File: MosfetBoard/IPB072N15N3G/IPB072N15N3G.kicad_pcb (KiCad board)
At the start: 2 copper layers, 147 x 100 mm, 94 parts, among them J1 DRIVER1, J13 BATT+Conn2, J14 BATT-Conn2, J2 DRIVER1, J3 DRIVER1, J4 PhaseConn, J5 PhaseConn, J6 PhaseConn, J8 BATT+Conn1, J9 BATT-Conn1, Q1 IPB072N15N3G, Q10 IPB072N15N3G, Q11 IPB072N15N3G, Q12 IPB072N15N3G, Q2 IPB072N15N3G, Q3 IPB072N15N3G, Q4 IPB072N15N3G, Q5 IPB072N15N3G, Q6 IPB072N15N3G, Q7 IPB072N15N3G, Q8 IPB072N15N3G, Q9 IPB072N15N3G, U1 RS2166XC5, U2 ACS773ECB-200B-PFF-T, U3 ACS773ECB-200B-PFF-T, U5 RS2166XC5, U6 ACS773ECB-200B-PFF-T, U7 RS2166XC5

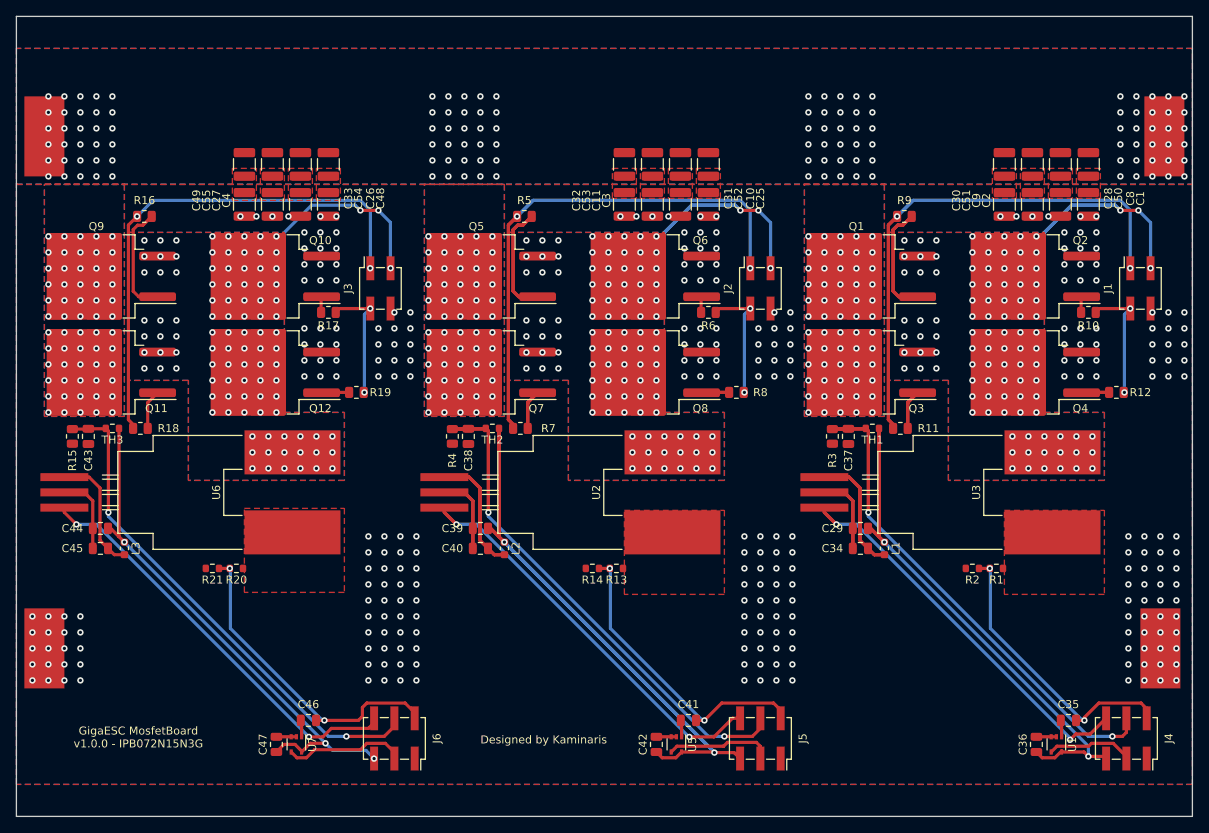
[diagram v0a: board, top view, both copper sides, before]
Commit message: v3.0.2 - IPB v2
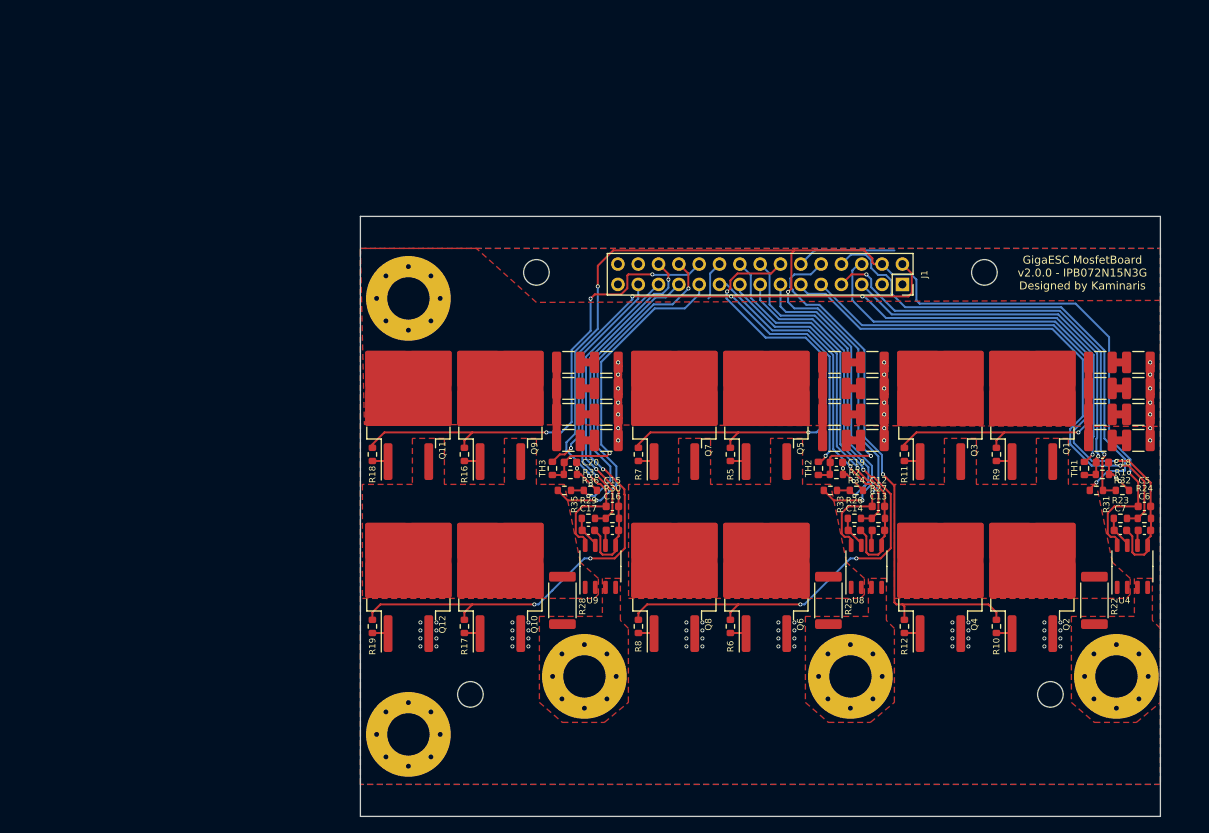
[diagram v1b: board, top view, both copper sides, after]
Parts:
- removed C29, C35, C36, C39, C41, C42, C44, C46, C47: 100nF, Capacitor_SMD:C_0805_2012Metric
- removed C34, C40, C45: 2.2u, Capacitor_SMD:C_0805_2012Metric
- removed C37, C38, C43: 1u, Capacitor_SMD:C_0805_2012Metric
- removed J13: BATT+Conn2, Connector_Wire:SolderWirePad_1x01_SMD_5x10mm
- removed J14: BATT-Conn2, Connector_Wire:SolderWirePad_1x01_SMD_5x10mm
- removed J2, J3: DRIVER1, Connector_PinSocket_2.54mm:PinSocket_2x02_P2.54mm_Vertical_SMD
- removed J4, J5, J6: PhaseConn, Connector_PinSocket_2.54mm:PinSocket_2x03_P2.54mm_Vertical_SMD
- removed J8: BATT+Conn1, Connector_Wire:SolderWirePad_1x01_SMD_5x10mm
- removed J9: BATT-Conn1, Connector_Wire:SolderWirePad_1x01_SMD_5x10mm
- removed L1, L2, L3: BLM18HE152SN1D, Inductor_SMD:L_0603_1608Metric
- removed R13, R20: 150k, Resistor_SMD:R_0603_1608Metric
- removed R14, R21: 2.7k, Resistor_SMD:R_0603_1608Metric
- removed R15, R4: 10k, Resistor_SMD:R_0805_2012Metric
- removed U1, U5, U7: RS2166XC5, Package_TO_SOT_SMD:SOT-353_SC-70-5
- removed U2, U3, U6: ACS773ECB-200B-PFF-T, GigaVescLibs:Allegro_CB_SMD
- added C12: 100n, Capacitor_SMD:C_0603_1608Metric, F.Cu at (170.8, 90.2)
- added C13: 10n, Capacitor_SMD:C_0603_1608Metric, F.Cu at (170.8, 93.2)
- added C14: 1n, Capacitor_SMD:C_0603_1608Metric, F.Cu at (167.8, 93.2)
- added C15: 100n, Capacitor_SMD:C_0603_1608Metric, F.Cu at (137.5, 90.2)
- added C16: 10n, Capacitor_SMD:C_0603_1608Metric, F.Cu at (137.5, 93.2)
- added C17: 1n, Capacitor_SMD:C_0603_1608Metric, F.Cu at (134.5, 93.2)
- added C18: 1u, Capacitor_SMD:C_0603_1608Metric, F.Cu at (198.8, 84.8)
- added C19: 1u, Capacitor_SMD:C_0603_1608Metric, F.Cu at (165.5, 84.8)
- added C20: 1u, Capacitor_SMD:C_0603_1608Metric, F.Cu at (132.2, 84.8)
- added C5: 100n, Capacitor_SMD:C_0603_1608Metric, F.Cu at (204.0, 90.2)
- added C6: 10n, Capacitor_SMD:C_0603_1608Metric, F.Cu at (204.0, 93.2)
- added C7: 1n, Capacitor_SMD:C_0603_1608Metric, F.Cu at (201.0, 93.2)
- added H1: MountingHole_Pad, MountingHole:MountingHole_5.3mm_M5_Pad_Via, F.Cu at (200.5, 111.5)
- added H2: MountingHole_Pad, MountingHole:MountingHole_5.3mm_M5_Pad_Via, F.Cu at (167.2, 111.5)
- added H3: MountingHole_Pad, MountingHole:MountingHole_5.3mm_M5_Pad_Via, F.Cu at (134.0, 111.5)
- added H4: MountingHole_Pad, MountingHole:MountingHole_5.3mm_M5_Pad_Via, F.Cu at (112.0, 118.8)
- added H5: MountingHole_Pad, MountingHole:MountingHole_5.3mm_M5_Pad_Via, F.Cu at (112.0, 64.2)
- added H6: MountingHole, MountingHole:MountingHole_3.2mm_M3_ISO14580, F.Cu at (128.0, 61.0)
- added H7: MountingHole, MountingHole:MountingHole_3.2mm_M3_ISO14580, F.Cu at (184.0, 61.0)
- added H8: MountingHole, MountingHole:MountingHole_3.2mm_M3_ISO14580, F.Cu at (119.8, 113.8)
- added H9: MountingHole, MountingHole:MountingHole_3.2mm_M3_ISO14580, F.Cu at (192.2, 113.8)
- added R22: 0.3m, Resistor_SMD:R_2512_6332Metric, F.Cu at (197.8, 102.0)
- added R23: 4.7k, Resistor_SMD:R_0603_1608Metric, F.Cu at (201.0, 91.8)
- added R24: 9.1k, Resistor_SMD:R_0603_1608Metric, F.Cu at (204.0, 91.8)
- added R25: 0.3m, Resistor_SMD:R_2512_6332Metric, F.Cu at (164.5, 102.0)
- added R26: 4.7k, Resistor_SMD:R_0603_1608Metric, F.Cu at (167.8, 91.8)
- added R27: 9.1k, Resistor_SMD:R_0603_1608Metric, F.Cu at (170.8, 91.8)
- added R28: 0.3m, Resistor_SMD:R_2512_6332Metric, F.Cu at (131.2, 102.0)
- added R29: 4.7k, Resistor_SMD:R_0603_1608Metric, F.Cu at (134.5, 91.8)
- added R30: 9.1k, Resistor_SMD:R_0603_1608Metric, F.Cu at (137.5, 91.8)
- added R31: 150k, Resistor_SMD:R_0603_1608Metric, F.Cu at (198.0, 88.2)
- added R32: 2.7k, Resistor_SMD:R_0603_1608Metric, F.Cu at (201.2, 88.2)
- added R33: 150k, Resistor_SMD:R_0603_1608Metric, F.Cu at (164.8, 88.2)
- added R34: 2.7k, Resistor_SMD:R_0603_1608Metric, F.Cu at (168.0, 88.2)
- added R35: 150k, Resistor_SMD:R_0603_1608Metric, F.Cu at (131.5, 88.2)
- added R36: 2.7k, Resistor_SMD:R_0603_1608Metric, F.Cu at (134.8, 88.2)
- added U4: MT9223CT-50BR5, Package_SO:SOP-8_3.9x4.9mm_P1.27mm, F.Cu at (202.5, 97.8)
- added U8: MT9223CT-50BR5, Package_SO:SOP-8_3.9x4.9mm_P1.27mm, F.Cu at (169.2, 97.8)
- added U9: MT9223CT-50BR5, Package_SO:SOP-8_3.9x4.9mm_P1.27mm, F.Cu at (136.0, 97.8)
- J1: value DRIVER1 -> LogicConnector; footprint Connector_PinSocket_2.54mm:PinSocket_2x02_P2.54mm_Vertical_SMD -> Connector_PinSocket_2.54mm:PinSocket_2x15_P2.54mm_Vertical
- Q1, Q10, Q11, Q12, Q2, Q3, Q4, Q5, Q6, Q7, Q8, Q9: footprint GigaVescLibs:TO-263-3_TabPin2_NoLeg -> Package_TO_SOT_SMD:TO-263-2
- R1: value 150k -> 10k
- R10, R11, R12, R16, R17, R18, R19, R3, R5, R6, R7, R8, R9: footprint Resistor_SMD:R_0805_2012Metric -> Resistor_SMD:R_0603_1608Metric
- R2: value 2.7k -> 10k
- moved TH3 55.2 mm to (130.0, 85.5), turned to -90 degrees
- moved C49 54.0 mm to (136.8, 82.0), turned to 0 degrees
- moved C33 53.2 mm to (132.0, 82.0), turned to 0 degrees
- moved Q9 52.8 mm to (123.5, 77.0), turned to 90 degrees
- moved R16 49.9 mm to (119.0, 83.8), turned to -90 degrees
- moved C55 49.3 mm to (136.8, 78.8), turned to 0 degrees
- moved C54 48.4 mm to (132.0, 78.8), turned to 0 degrees
- moved Q10 47.6 mm to (123.5, 98.5), turned to 90 degrees
- moved C27 44.6 mm to (136.8, 75.5), turned to 0 degrees
- moved C26 43.7 mm to (132.0, 75.5), turned to 0 degrees
- moved C31 43.4 mm to (165.2, 82.0), turned to 0 degrees
- moved C32 42.8 mm to (170.0, 82.0), turned to 0 degrees
- moved R17 42.8 mm to (119.0, 105.2), turned to -90 degrees
- moved TH2 41.1 mm to (163.2, 85.5), turned to -90 degrees
- moved R10 40.9 mm to (185.5, 105.2), turned to -90 degrees
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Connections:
- J1 pad 1: /PhaseMosfets1/PH -> Net-(J1-Pin_1)
- J1 pad 2: /PhaseMosfets1/PL -> /3.3V
- J1 pad 3: /PhaseMosfets1/PHASE -> unconnected-(J1-Pin_3-Pad3)
- J1 pad 4: -BATT -> /5V
- Q1 pad 3: /PhaseMosfets1/PHASE -> /PHASE1
- Q10 pad 2: /PhaseMosfets3/PHASE -> /PHASE3
- Q11 pad 3: /PhaseMosfets3/PHASE -> /PHASE3
- Q12 pad 2: /PhaseMosfets3/PHASE -> /PHASE3
- Q2 pad 2: /PhaseMosfets1/PHASE -> /PHASE1
- Q3 pad 3: /PhaseMosfets1/PHASE -> /PHASE1
- Q4 pad 2: /PhaseMosfets1/PHASE -> /PHASE1
- Q5 pad 3: /PhaseMosfets2/PHASE -> /PHASE2
- Q6 pad 2: /PhaseMosfets2/PHASE -> /PHASE2
- Q7 pad 3: /PhaseMosfets2/PHASE -> /PHASE2
- Q8 pad 2: /PhaseMosfets2/PHASE -> /PHASE2
- Q9 pad 3: /PhaseMosfets3/PHASE -> /PHASE3
- R1 pad 1: /PhaseMosfets1/PHASE_OUT -> /PhaseMosfets1/MOS_TEMP
- R1 pad 2: /PhaseMosfets1/V_SENSE -> -BATT
- R10 pad 1: /PhaseMosfets1/PL -> /PL1
- R11 pad 1: /PhaseMosfets1/PH -> /PH1
- R12 pad 1: /PhaseMosfets1/PL -> /PL1
- R16 pad 1: /PhaseMosfets3/PH -> /PH3
- R17 pad 1: /PhaseMosfets3/PL -> /PL3
- R18 pad 1: /PhaseMosfets3/PH -> /PH3
- R19 pad 1: /PhaseMosfets3/PL -> /PL3
- R2 pad 1: /PhaseMosfets1/V_SENSE -> /PhaseMosfets2/MOS_TEMP
- R3 pad 1: /PhaseMosfets1/MOS_TEMP -> /PhaseMosfets3/MOS_TEMP
- R5 pad 1: /PhaseMosfets2/PH -> /PH2
- R6 pad 1: /PhaseMosfets2/PL -> /PL2
- R7 pad 1: /PhaseMosfets2/PH -> /PH2
- R8 pad 1: /PhaseMosfets2/PL -> /PL2
- R9 pad 1: /PhaseMosfets1/PH -> /PH1
- TH1 pad 1: /PhaseMosfets1/3.3V_IN -> /3.3V
- TH2 pad 1: /PhaseMosfets2/3.3V_IN -> /3.3V
- TH3 pad 1: /PhaseMosfets3/3.3V_IN -> /3.3V
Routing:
- net /5V: track 0.00 -> 193.8 mm, vias 0 -> 5
- net /3.3V: track 0.00 -> 139.6 mm, vias 0 -> 6
- net /PhaseMosfets2/PH: track 119.9 -> 0.00 mm, vias 2 -> 0
- net /PhaseMosfets1/PH: track 119.9 -> 0.00 mm, vias 2 -> 0
- net /PhaseMosfets2/3.3V_IN: track 118.0 -> 0.00 mm, vias 2 -> 0
- net /PL2: track 0.00 -> 84.2 mm, vias 0 -> 3
- net /PL3: track 0.00 -> 80.7 mm, vias 0 -> 4
- net /PhaseMosfets1/3.3V_IN: track 79.8 -> 0.00 mm, vias 2 -> 0
- net /PhaseMosfets1/SH-: track 0.00 -> 73.9 mm, vias 0 -> 1
- net /PH1: track 0.00 -> 73.1 mm, vias 0 -> 1
- net /PhaseMosfets1/SH+: track 0.00 -> 68.1 mm, vias 0 -> 1
- net /PL1: track 0.00 -> 67.6 mm, vias 0 -> 1
- net /PhaseMosfets3/3.3V_IN: track 66.2 -> 0.00 mm, vias 3 -> 0
- net /PhaseMosfets3/PH: track 64.4 -> 0.00 mm, vias 2 -> 0
- net /PH3: track 0.00 -> 61.6 mm, vias 0 -> 3
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- added copper zone on F.Cu, net /PHASE1
- added copper zone on F.Cu, net /PHASE2
- added copper zone on F.Cu, net /PHASE3
- removed copper zone on B.Cu, net +BATT
- removed copper zone on B.Cu, net /PhaseMosfets1/PHASE
- removed copper zone on F.Cu, net /PhaseMosfets1/PHASE
- removed copper zone on B.Cu, net /PhaseMosfets2/PHASE
- removed copper zone on F.Cu, net /PhaseMosfets2/PHASE
- removed copper zone on B.Cu, net /PhaseMosfets3/PHASE
- removed copper zone on F.Cu, net /PhaseMosfets3/PHASE
- removed copper zone on F.Cu, net Net-(C1-Pad2)
- removed copper zone on F.Cu, net Net-(C10-Pad2)
- removed copper zone on F.Cu, net Net-(C25-Pad2)
- removed copper zone on F.Cu, net Net-(C26-Pad2)
- removed copper zone on F.Cu, net Net-(C28-Pad2)
- removed copper zone on F.Cu, net Net-(C31-Pad2)
- removed copper zone on F.Cu, net Net-(C33-Pad2)
- removed copper zone on F.Cu, net Net-(C4-Pad1)
- removed copper zone on F.Cu, net Net-(C50-Pad2)
- removed copper zone on F.Cu, net Net-(C52-Pad2)
- removed copper zone on F.Cu, net Net-(C54-Pad2)
- removed copper zone on F.Cu, net Net-(C8-Pad2)
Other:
- board size 147 x 100 mm -> 100 x 75 mm
- board text added: "GigaESC MosfetBoard v2.0.0 - IPB072N15N3G Designed by Kaminaris"
- board text removed: "Designed by Kaminaris"
- board text removed: "GigaESC MosfetBoard v1.0.0 - IPB072N15N3G"
